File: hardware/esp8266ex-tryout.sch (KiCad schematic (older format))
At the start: 21 parts, among them U1 ESP8266EX, U2 W25Q32JVSSIQ, U3 ESP8266EX_SERVICE, Y1 O_26M,3225

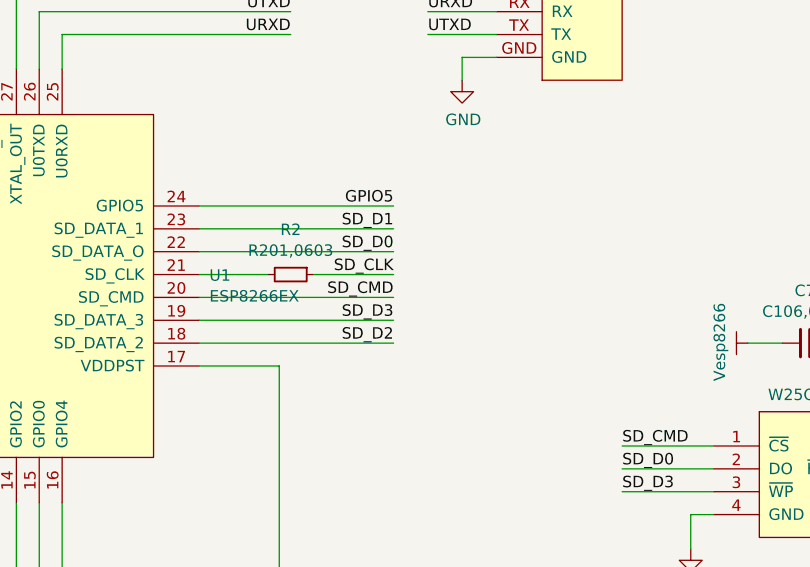
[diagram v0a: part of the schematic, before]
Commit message: update for RN,
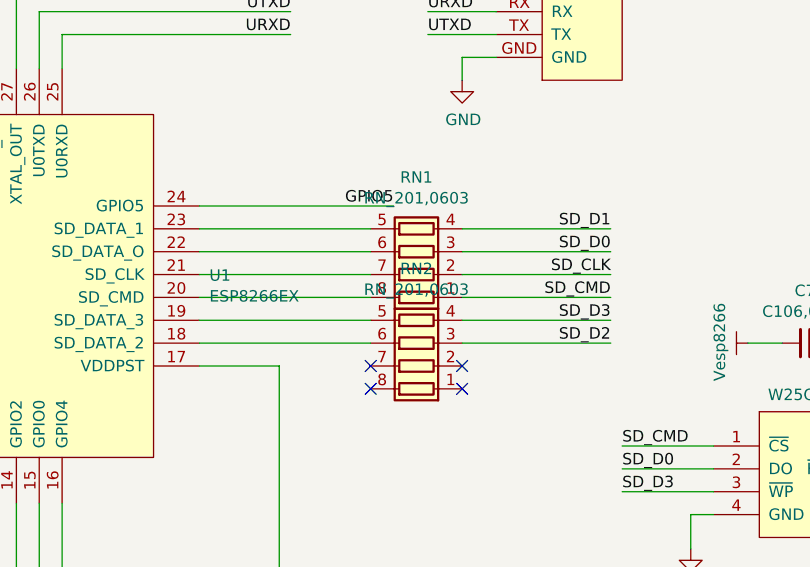
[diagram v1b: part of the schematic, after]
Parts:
- removed R2: R201,0603, Resistor_SMD:R_0603_1608Metric_Pad1.05x0.95mm_HandSolder, symbol taobao-r:R201,0603
- added RN1, RN2: RN_201,0603, Resistor_SMD:R_Array_Concave_4x0603, symbol taobao-rpack:RN_201,0603
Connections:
- net SD_CLK: now also RN1.2 (R2.1)
- net SD_CMD: now also RN1.1 (R1.1); no longer U1.20 (SD_CMD)
- net SD_D0: now also RN1.3 (R3.1); no longer U1.22 (SD_DATA_O)
- net SD_D1: now also RN1.4 (R4.1); no longer U1.23 (SD_DATA_1)
- net SD_D2: now also RN2.3 (R3.1); no longer U1.18 (SD_DATA_2)
- net SD_D3: now also RN2.4 (R4.1); no longer U1.19 (SD_DATA_3)
- net at U1.21 (SD_CLK): now also RN1.7 (R2.2)
- new net: RN2.6 (R3.2), U1.18 (SD_DATA_2)
- new net: RN2.5 (R4.2), U1.19 (SD_DATA_3)
- new net: RN1.8 (R1.2), U1.20 (SD_CMD)
- new net: RN1.6 (R3.2), U1.22 (SD_DATA_O)
- new net: RN1.5 (R4.2), U1.23 (SD_DATA_1)
- no-connect marks 1 -> 5
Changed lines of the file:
@@
 Text Label 8250 2650 2    50   ~ 0
 GPIO5
-Text Label 8250 2750 2    50   ~ 0
+Text Label 9200 2750 2    50   ~ 0
 SD_D1
-Text Label 8250 2850 2    50   ~ 0
+Text Label 9200 2850 2    50   ~ 0
 SD_D0
-Text Label 8250 2950 2    50   ~ 0
+Text Label 9200 2950 2    50   ~ 0
 SD_CLK
-Text Label 8250 3050 2    50   ~ 0
+Text Label 9200 3050 2    50   ~ 0
 SD_CMD
-Text Label 8250 3150 2    50   ~ 0
+Text Label 9200 3150 2    50   ~ 0
 SD_D3
-Text Label 8250 3250 2    50   ~ 0
+Text Label 9200 3250 2    50   ~ 0
 SD_D2
 Wire Wire Line
 	7400 2650 8250 2650
-Wire Wire Line
-	7400 2750 8250 2750
-Wire Wire Line
-	7400 2850 8250 2850
-Wire Wire Line
-	7400 3050 8250 3050
-Wire Wire Line
-	7400 3150 8250 3150
-Wire Wire Line
-	7400 3250 8250 3250
 Text Label 7800 1700 2    50   ~ 0
 RST
@@
 Connection ~ 6950 1250
 $Comp
-L taobao-r:R201,0603 R2
-U 1 1 5D014F86
-P 7800 2950
-F 0 "R2" V 7604 2950 50  0000 C CNN
-F 1 "R201,0603" V 7695 2950 50  0000 C CNN
-F 2 "Resistor_SMD:R_0603_1608Metric_Pad1.05x0.95mm_HandSolder" H 7800 2950 50  0001 C CNN
-F 3 "~" H 7800 2950 50  0001 C CNN
-	1    7800 2950
-	0    1    1    0
-$EndComp
-Wire Wire Line
-	7400 2950 7700 2950
-Wire Wire Line
-	7900 2950 8250 2950
-$Comp
 L my_power:Vesp8266 #PWR0114
 U 1 1 5D020F93
@@
 Wire Wire Line
 	8550 2000 8700 2000
+$Comp
+L taobao-rpack:RN_201,0603 RN1
+U 1 1 5CFCF99C
+P 8350 2850
+F 0 "RN1" V 8675 2850 50  0000 C CNN
+F 1 "RN_201,0603" V 8584 2850 50  0000 C CNN
+F 2 "Resistor_SMD:R_Array_Concave_4x0603" V 8625 2850 50  0001 C CNN
+F 3 "~" H 8350 2850 50  0001 C CNN
+	1    8350 2850
+	0    -1   -1   0
+$EndComp
+$Comp
+L taobao-rpack:RN_201,0603 RN2
+U 1 1 5CFEBB7D
+P 8350 3250
+F 0 "RN2" V 8675 3250 50  0000 C CNN
+F 1 "RN_201,0603" V 8584 3250 50  0000 C CNN
+F 2 "Resistor_SMD:R_Array_Concave_4x0603" V 8625 3250 50  0001 C CNN
+F 3 "~" H 8350 3250 50  0001 C CNN
+	1    8350 3250
+	0    -1   -1   0
+$EndComp
+Wire Wire Line
+	8550 3250 9200 3250
+Wire Wire Line
+	8550 2750 9200 2750
+Wire Wire Line
+	7400 2750 8150 2750
+Wire Wire Line
+	8550 2850 9200 2850
+Wire Wire Line
+	8550 3050 9200 3050
+Wire Wire Line
+	8550 3150 9200 3150
+Wire Wire Line
+	8550 2950 9200 2950
+Wire Wire Line
+	7400 2850 8150 2850
+Wire Wire Line
+	7400 2950 8150 2950
+Wire Wire Line
+	7400 3050 8150 3050
+Wire Wire Line
+	7400 3150 8150 3150
+Wire Wire Line
+	7400 3250 8150 3250
+NoConn ~ 8150 3350
+NoConn ~ 8150 3450
+NoConn ~ 8550 3450
+NoConn ~ 8550 3350
 $EndSCHEMATC
